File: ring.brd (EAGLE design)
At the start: 83.1 x 90 mm, 22 parts

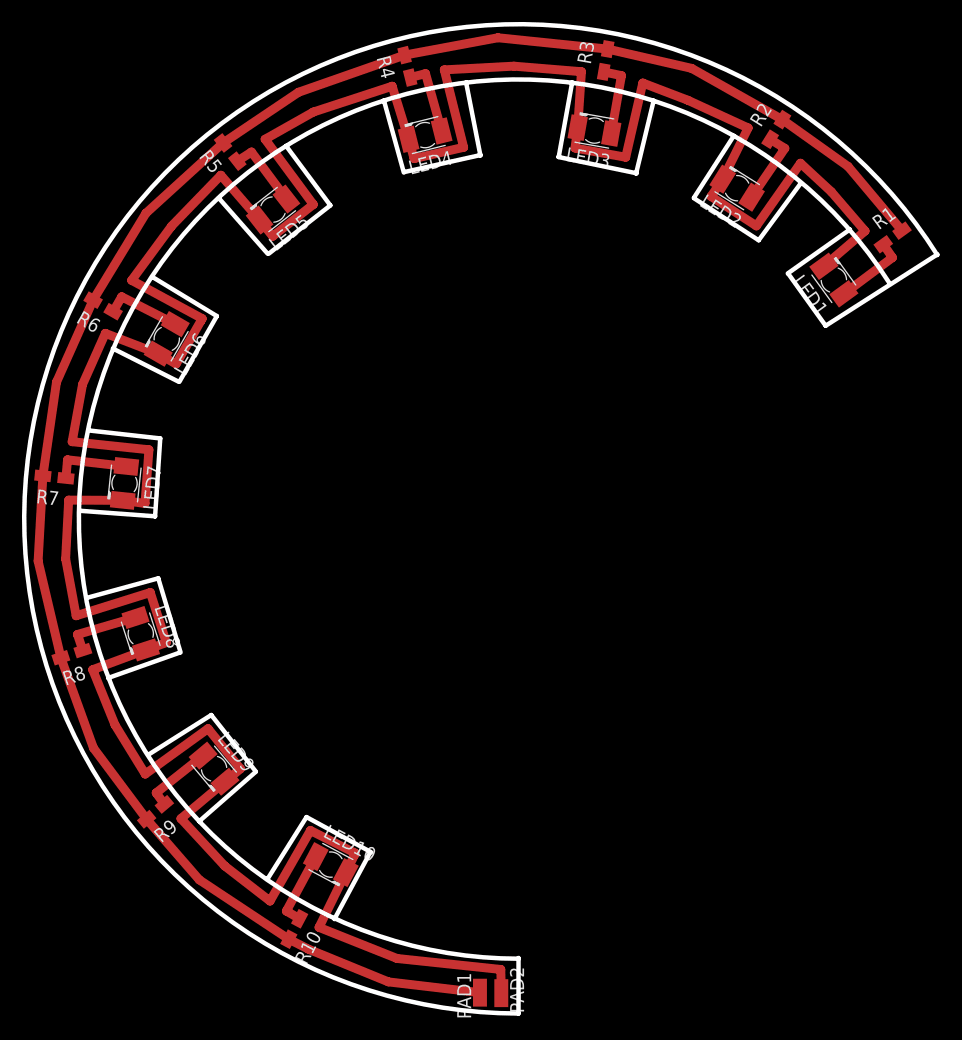
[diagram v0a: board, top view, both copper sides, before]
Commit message: curve
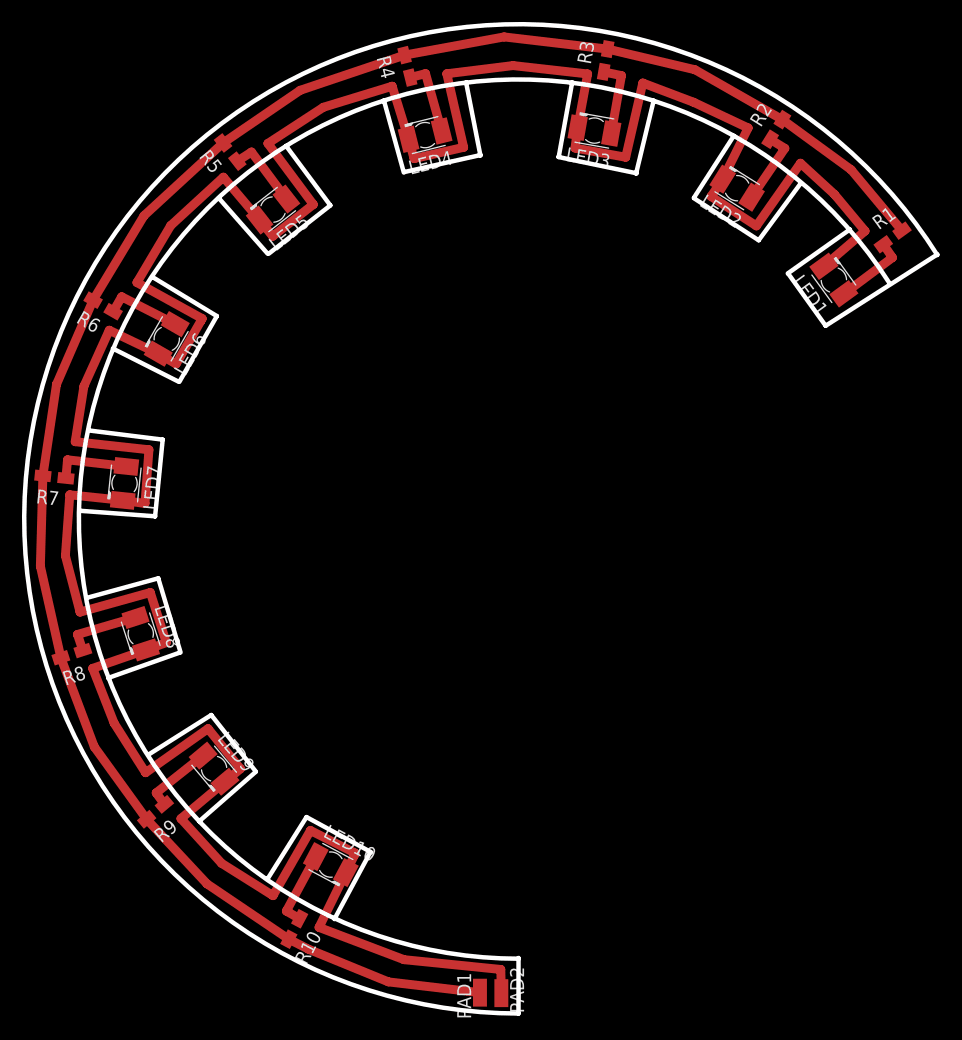
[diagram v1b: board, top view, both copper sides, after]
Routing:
- net N$2: track 294.6 -> 291.9 mm
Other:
- outline, holes or cut-outs redrawn

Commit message: new
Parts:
- added LED11, LED12, LED13, LED14, LED15, LED16: (no value), led:KA-3528ASYC
- added PAD3, PAD4: (no value), wirepad:SMD1,27-2,54
- added R11, R12, R13, R14, R15, R16: 330R, rcl:R0805W
- moved LED3 200.3 mm to (-90.0, -140.0), turned to 0 degrees
- moved LED1 189.6 mm to (-85.0, -130.0), turned to 0 degrees
- moved LED4 189.0 mm to (-80.0, -140.0), turned to 0 degrees
- moved LED2 186.1 mm to (-75.0, -130.0), turned to 0 degrees
- moved R1 176.5 mm to (-90.0, -100.0), turned to 0 degrees
- moved LED5 174.8 mm to (-70.0, -140.0), turned to 0 degrees
- moved LED6 171.5 mm to (-90.0, -145.0), turned to 0 degrees
- moved R4 171.0 mm to (-90.0, -110.0), turned to 0 degrees
- moved R2 170.4 mm to (-80.0, -100.0), turned to 0 degrees
- moved R3 161.7 mm to (-70.0, -100.0), turned to 0 degrees
- moved LED7 154.7 mm to (-80.0, -145.0), turned to 0 degrees
- moved R5 153.1 mm to (-80.0, -110.0), turned to 0 degrees
- moved LED8 139.2 mm to (-70.0, -145.0), turned to 0 degrees
- moved R6 133.3 mm to (-70.0, -110.0), turned to 0 degrees
- moved R7 132.7 mm to (-90.0, -120.0), turned to 0 degrees
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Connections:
- new net N$11: PAD3.1, R10.2, R11.2, R12.2, R13.2, R14.2, R15.2, R16.2, R9.2
- new net N$12: LED10.C, LED11.C, LED12.C, LED13.C, LED14.C, LED15.C, LED16.C, LED9.C, PAD4.1
- new net N$15: LED11.A, R11.1
- new net N$16: LED12.A, R12.1
- new net N$17: LED13.A, R13.1
- new net N$18: LED14.A, R14.1
- new net N$19: LED15.A, R15.1
- new net N$20: LED16.A, R16.1
- net N$1: no longer R10.2, R9.2
- net N$2: no longer LED10.C, LED9.C
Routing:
- net N$2: track 291.9 -> 0.00 mm
- net N$1: track 173.8 -> 0.00 mm
- net N$9: track 7.07 -> 0.00 mm
- net N$10: track 7.04 -> 0.00 mm
- net N$8: track 7.04 -> 0.00 mm
- net N$14: track 7.03 -> 0.00 mm
- net N$5: track 7.00 -> 0.00 mm
- net N$3: track 6.98 -> 0.00 mm
- net N$4: track 6.95 -> 0.00 mm
- net N$7: track 6.87 -> 0.00 mm
- net N$6: track 6.86 -> 0.00 mm
- net N$13: track 6.74 -> 0.00 mm
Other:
- board size 83.1 x 90 mm -> 174.9 x 190 mm
